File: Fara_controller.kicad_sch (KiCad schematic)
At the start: 97 parts, among them U3 TPS61165DBV, U4 TPS61165DBV, U6 TPS61165DBV, U7 TPS61165DBV, U8 TPS563200, U9 TPS563200, X1 Conn_01x02, X10 Conn_01x02, X11 Conn_01x02, X12 Conn_01x02, X13 Conn_01x02, X14 Conn_01x02, X15 Conn_01x02, X16 Conn_01x02, X18 Objective, X19 Conn_01x02, X2 Conn_01x02, X20 Conn_01x03, X21 Conn_01x03, X3 Conn_01x02, X4 Conn_01x02, X5 Fan_3pin, X6 Fan_3pin, X7 Fan_3pin, X8 Fan_3pin, X9 Conn_01x02

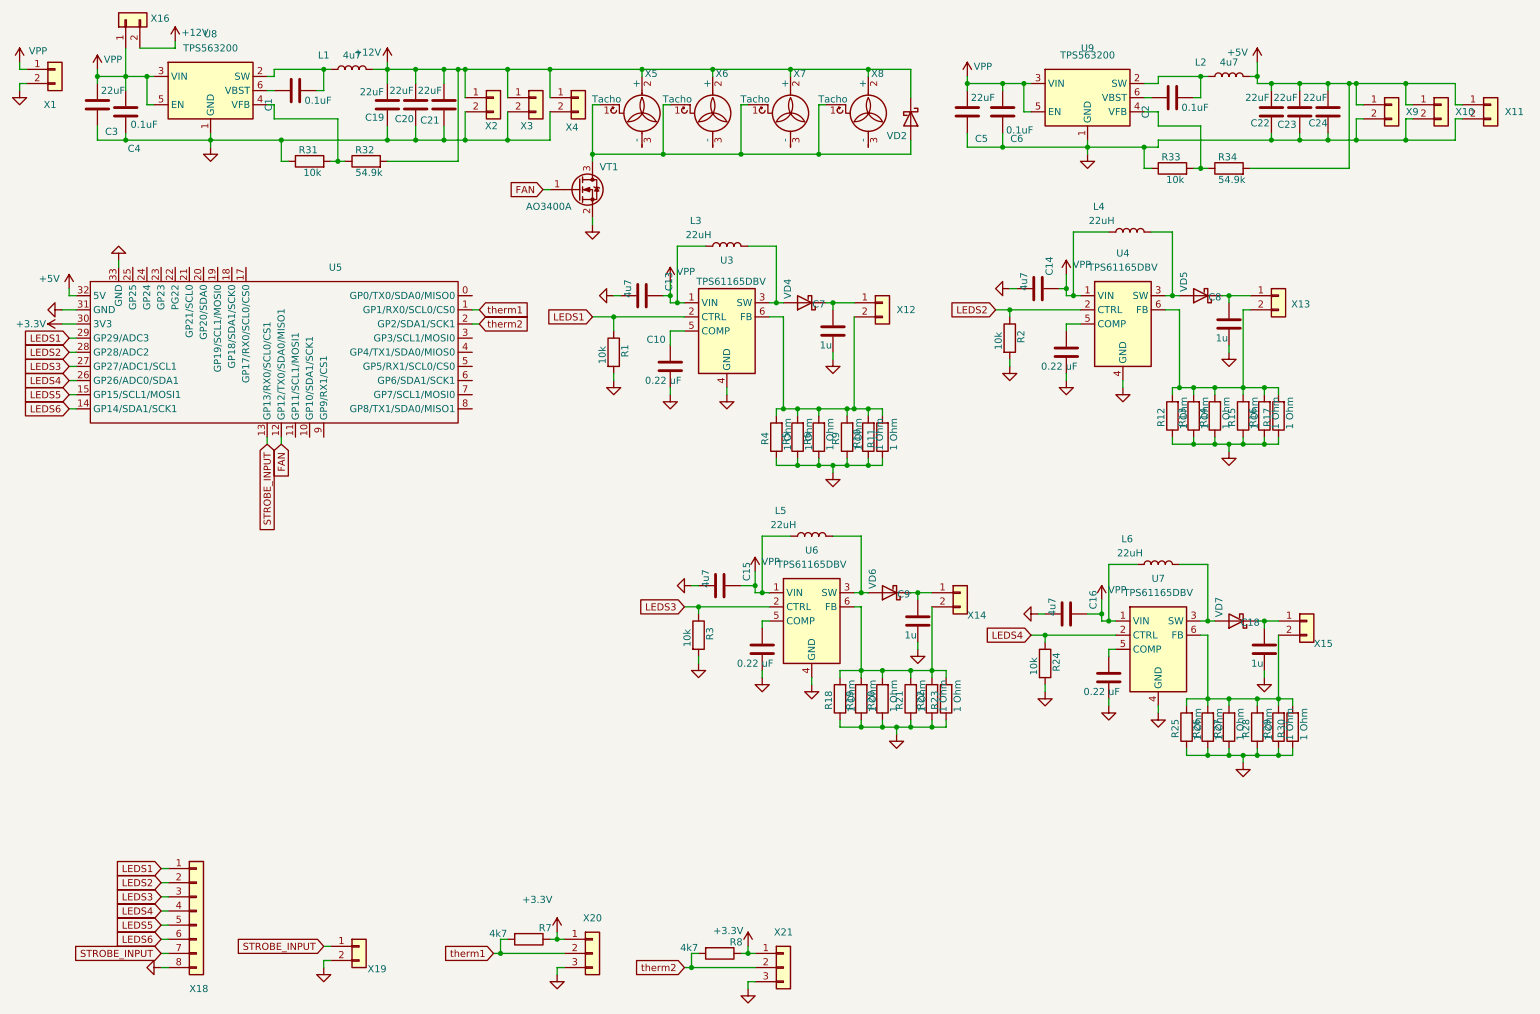
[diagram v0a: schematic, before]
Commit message: v0.9 small changes
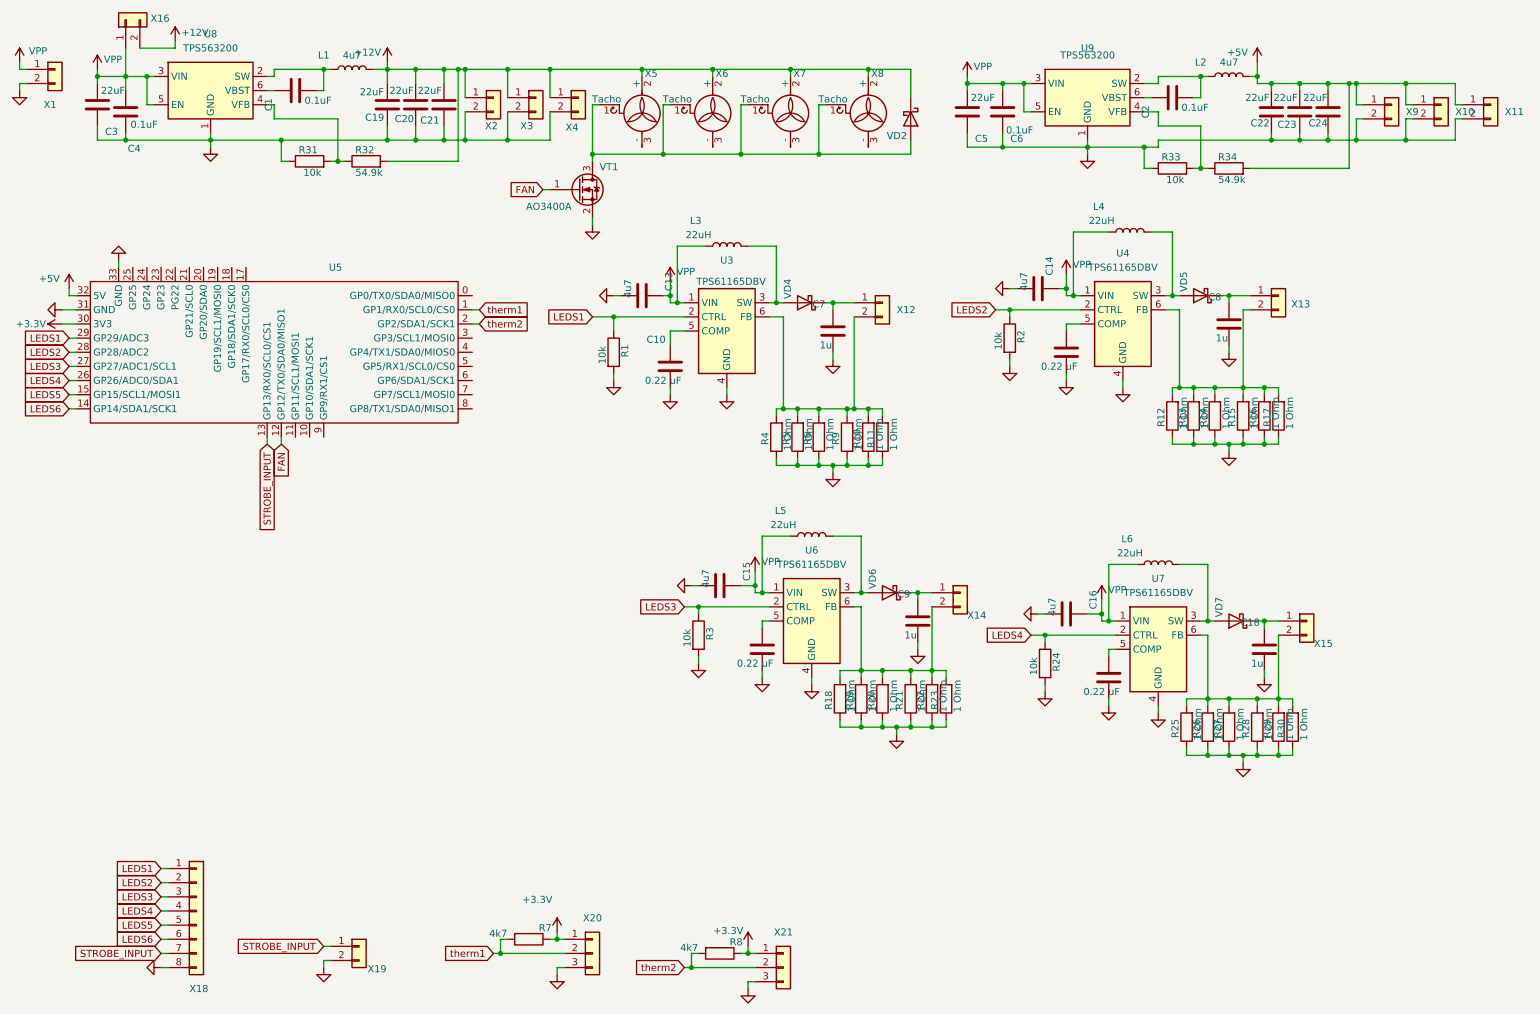
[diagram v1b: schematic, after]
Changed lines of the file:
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@@
 (kicad_sch
-	(version 20231120)
+	(version 20250114)
 	(generator "eeschema")
-	(generator_version "8.0")
+	(generator_version "9.0")
 	(paper "A4")
 	(junction
@@
 		)
 	)
+	(embedded_fonts no)
 )
